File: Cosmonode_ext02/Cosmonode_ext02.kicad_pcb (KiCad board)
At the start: 2 copper layers, 24.1 x 34.3 mm, 21 parts, among them J1 CONN_01X04, J2 CONN_01X04, J3 CONN_01X08, J4 CONN_01X08, J5 GS3, J6 GS3, J7 Aloes_Logo, J8 OSHW_Logo, Q1 BSS138, Q2 BSS138, SW1 SW_Push, SW2 SW_Push, U1 XC6206P502MR

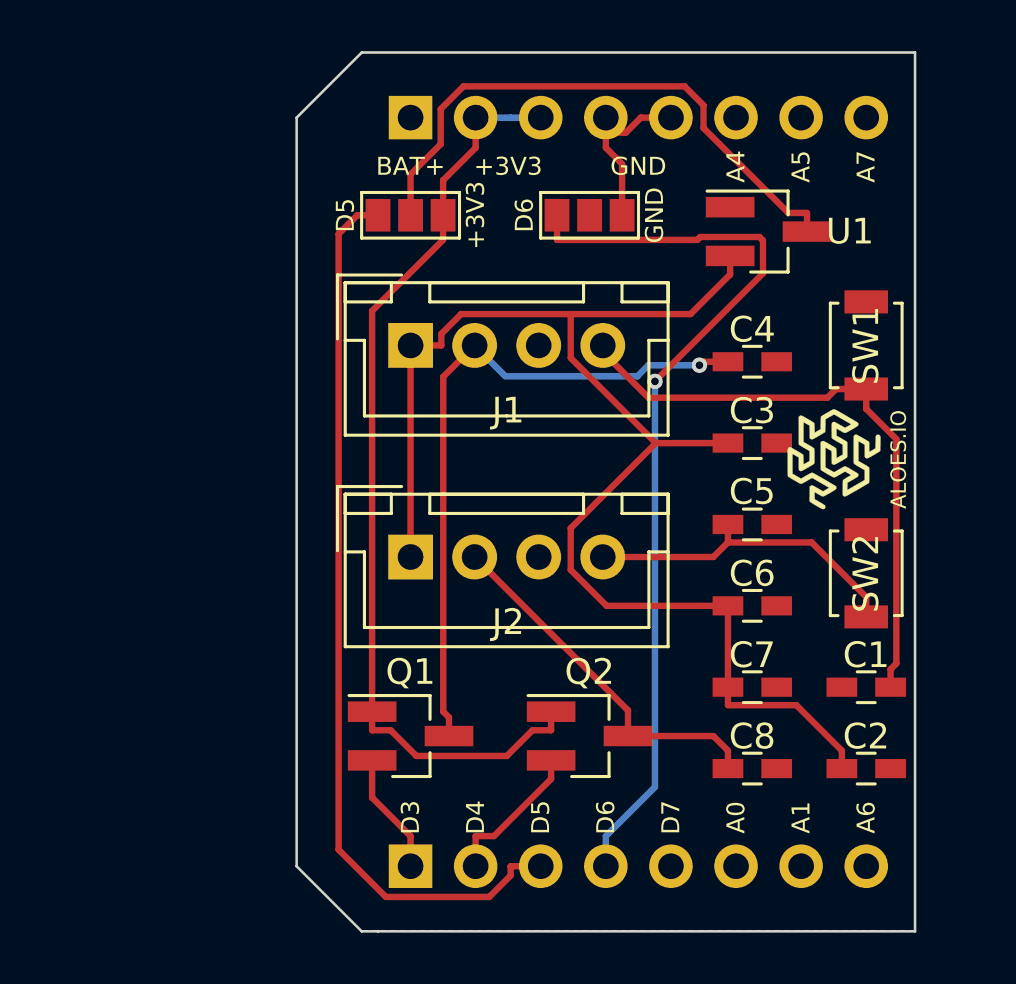
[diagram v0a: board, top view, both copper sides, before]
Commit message: update to V0.7 (WIP)
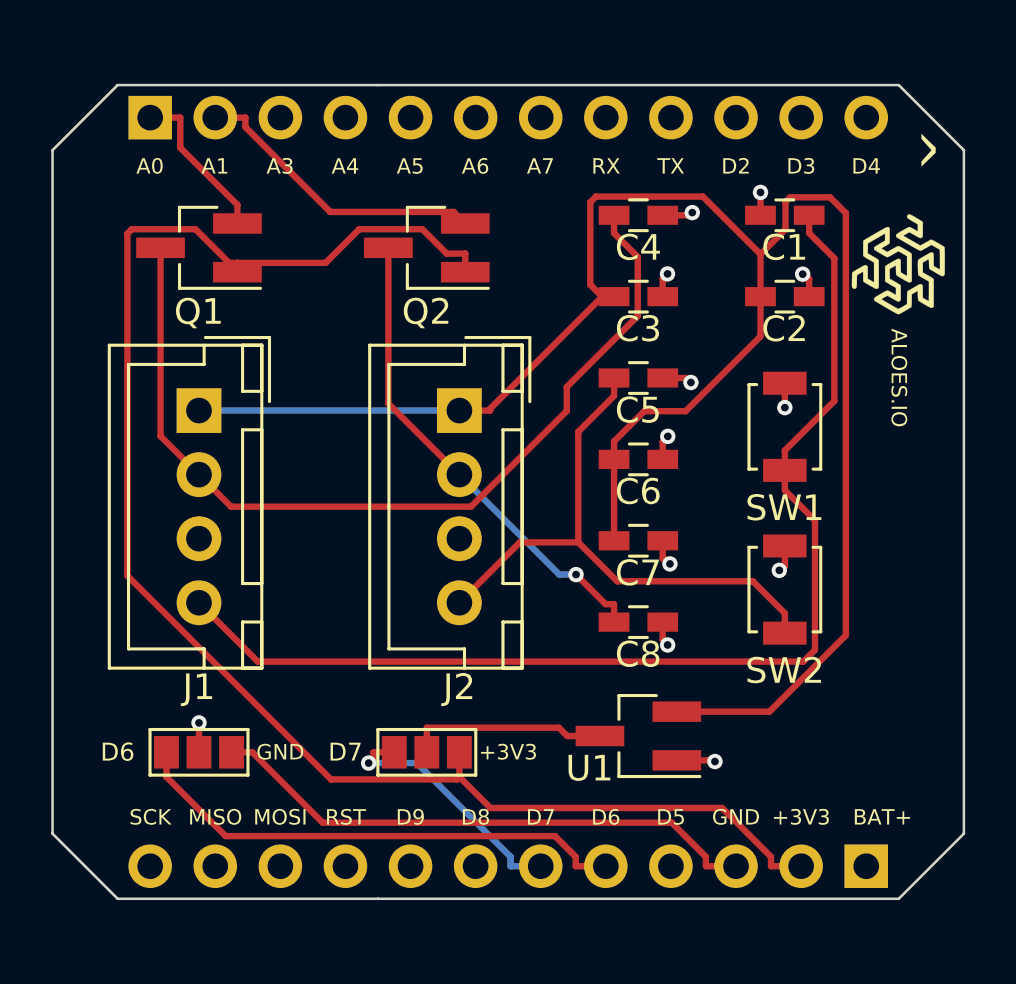
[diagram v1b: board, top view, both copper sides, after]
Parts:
- J3, J4: value CONN_01X08 -> CONN_01X12; footprint Pin_Headers:Pin_Header_Straight_1x08_Pitch2.54mm -> Socket_Strips:Socket_Strip_Straight_1x12_Pitch2.54mm
- moved J4 34.2 mm to (176.5, 120.7), turned to 90 degrees
- moved J3 30.9 mm to (148.6, 91.4)
- moved J6 25.9 mm to (150.5, 116.2)
- moved J5 21.0 mm to (159.4, 116.2)
- moved Q1 20.8 mm to (150.5, 96.5), turned to 180 degrees
- moved U1 20.3 mm to (167.6, 115.6), turned to 180 degrees
- moved Q2 20.1 mm to (159.4, 96.5), turned to 180 degrees
- moved C1 18.7 mm to (173.4, 95.2)
- moved C2 18.7 mm to (173.4, 98.4)
- moved J8 14.7 mm to (175.3, 97.8), turned to 90 degrees
- moved J1 8.64 mm to (150.5, 102.9), turned to 270 degrees
- moved J7 8.03 mm to (177.8, 97.2), turned to 270 degrees
- moved C3 7.24 mm to (167.6, 98.4)
- moved C4 7.24 mm to (167.6, 95.2)
- moved C5 7.24 mm to (167.6, 101.6)
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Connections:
- net /A0 renamed A6
- net /A1 renamed A7
- net /A5 renamed D8
- net /A6 renamed RX
- net /A7 renamed D9
- net /BAT+ renamed +BATT
- net /D3 renamed A0
- net /D3_5V renamed A0_5V
- net /D4 renamed A1
- net /D4_5V renamed A1_5V
- net /D7 renamed A5
- J3 pad 3: /D5 -> A3
- J3 pad 4: /D6 -> A4
- J4 pad 3: +3V3 -> GND
- J4 pad 4: GND -> D5
- J4 pad 5: GND -> D6
- J4 pad 6: /A4 -> D7
- J5 pad 1: /D5 -> D7
- J6 pad 1: /D6 -> D6
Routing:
- net /D6: track 36.1 -> 0.00 mm, vias 1 -> 0
- net /D5: track 35.2 -> 0.00 mm
- net +3V3: track 36.7 -> 61.4 mm
- net Net-(C1-Pad2): track 23.6 -> 43.8 mm
- net D6: track 0.00 -> 19.8 mm
- net +5V: track 54.9 -> 73.5 mm
- net GND: track 6.86 -> 21.7 mm
- net Net-(J5-Pad2): track 22.6 -> 7.85 mm
- net Net-(C1-Pad1): track 0.00 -> 12.9 mm, vias 0 -> 12
- net D7: track 0.00 -> 9.91 mm, vias 0 -> 1
- net Net-(C5-Pad2): track 12.9 -> 22.6 mm
- net A0_5V: track 26.5 -> 35.1 mm, vias 1 -> 0
- net A1: track 5.77 -> 11.7 mm
- net A1_5V: track 14.3 -> 18.8 mm, vias 0 -> 1
- net A0: track 4.75 -> 6.23 mm
- added copper zone on B.Cu, net Net-(C1-Pad1)
- removed copper zone on F.Cu, net Net-(C1-Pad1)
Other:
- board size 24.1 x 34.3 mm -> 35.6 x 31.8 mm
- board text added: "A3"
- board text added: "D2"
- board text added: "D8"
- board text added: "D9"
- board text added: "MISO"
- board text added: "MOSI"
- board text added: "RST"
- board text added: "RX"
- board text added: "SCK"
- board text added: "TX"
- board text added: "^"
